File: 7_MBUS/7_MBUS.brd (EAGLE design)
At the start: 67.4 x 44.8 mm, 23 parts, among them T1 BCP51-16, T2 BC847, T3 BC847, X1 AKL18X-02W, X12 ALLSERIALD

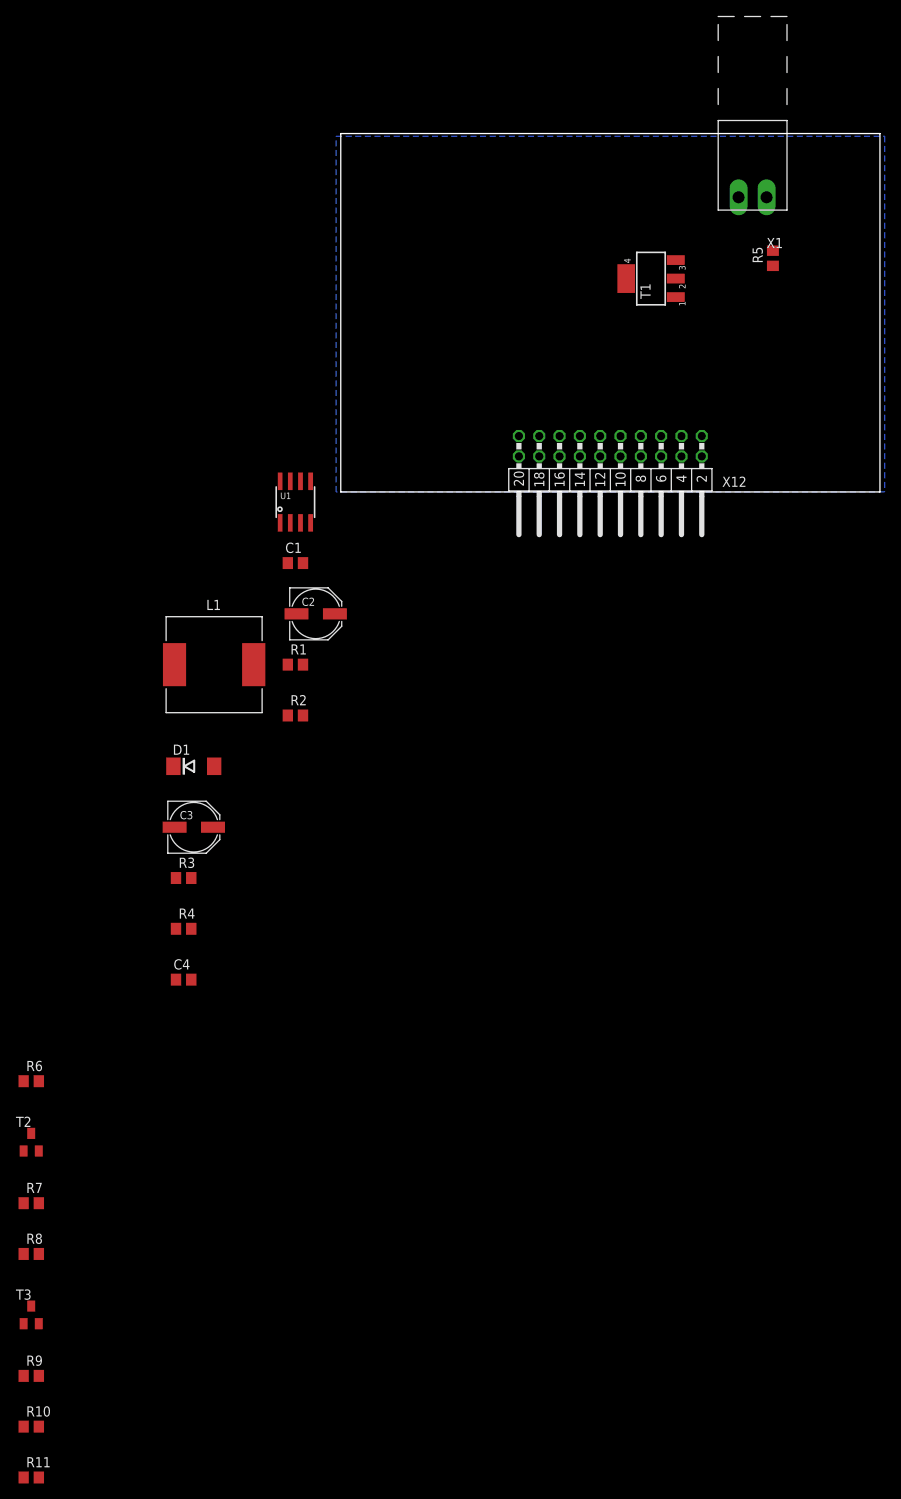
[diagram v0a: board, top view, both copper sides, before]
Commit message: change diodes
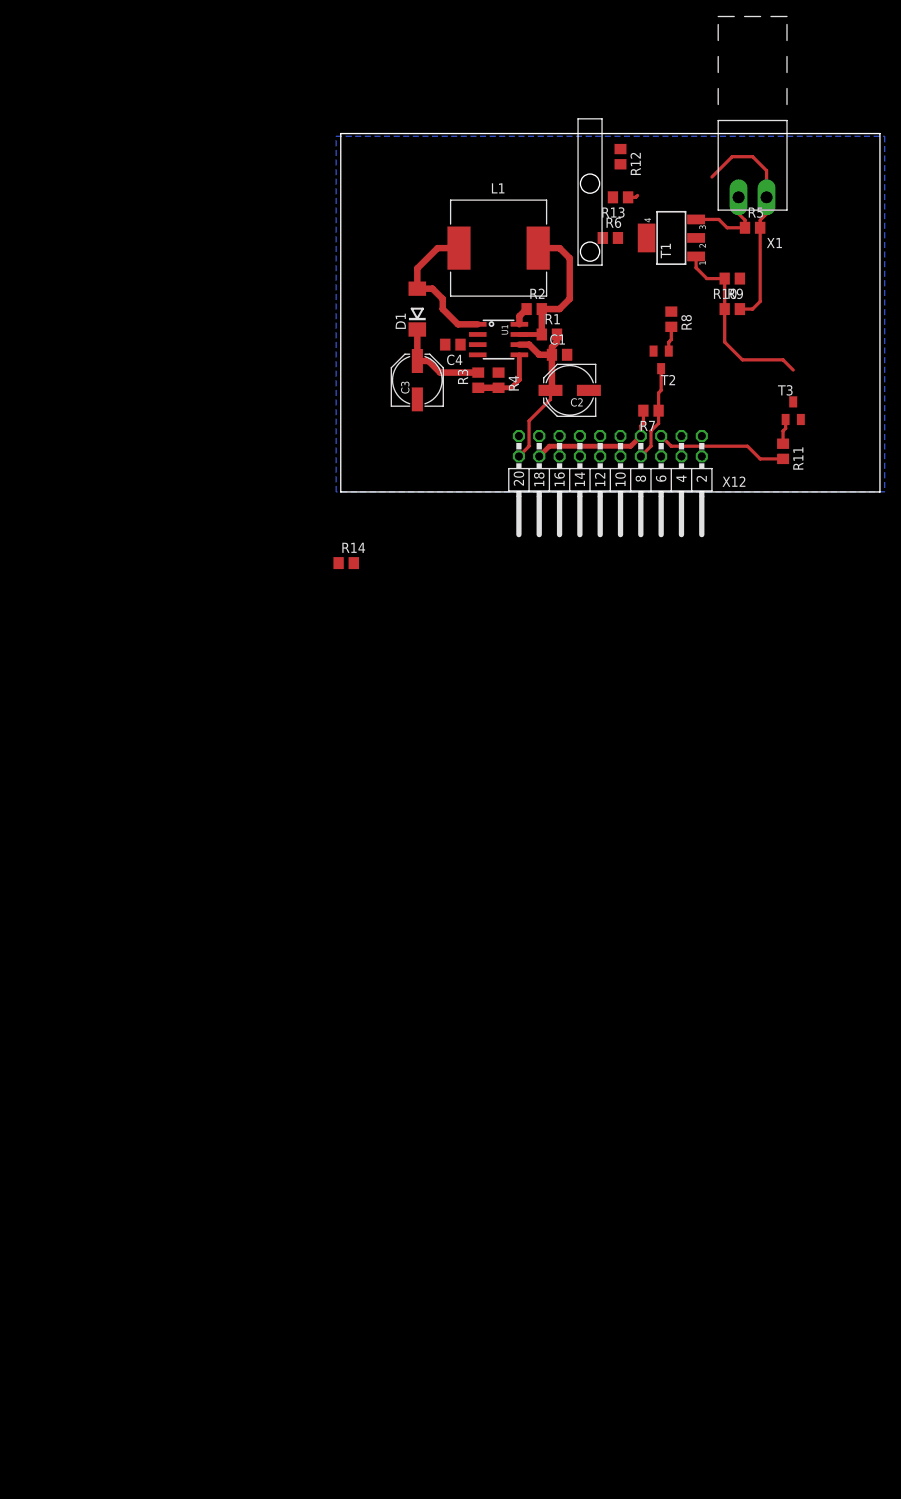
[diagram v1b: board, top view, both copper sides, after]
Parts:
- added R12: 39k, rcl:R0805
- added R13: 22, rcl:R0805
- added R14: 2k2, rcl:R0805
- added U$1: (no value), Mentor:1271.1000
- moved R10 168.1 mm to (15.2, 26.7), turned to 180 degrees
- moved R9 159.6 mm to (15.2, 22.9)
- moved R11 159.0 mm to (21.6, 5.08), turned to 270 degrees
- moved T3 147.8 mm to (22.9, 10.2)
- moved R8 141.6 mm to (7.62, 21.6), turned to 270 degrees
- moved R6 127.9 mm to (0.00, 31.8)
- moved R7 125.8 mm to (5.08, 10.2), turned to 180 degrees
- moved T2 125.6 mm to (6.35, 16.5), turned to 180 degrees
- moved C4 86.2 mm to (-19.7, 18.4), turned to 180 degrees
- moved R4 79.1 mm to (-14.0, 14.0), turned to 270 degrees
- moved R3 72.3 mm to (-16.5, 14.0), turned to 90 degrees
- moved D1 63.6 mm to (-24.1, 22.9), turned to 90 degrees
- moved L1 63.1 mm to (-14.0, 30.5)
- moved C3 62.5 mm to (-24.1, 14.0), turned to 90 degrees
- moved R2 58.9 mm to (-9.53, 22.9)
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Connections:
- new net N$100: R5.2, R9.2, X1.P$1
- new net N$11: R13.1
- new net N$14: R14.2, T3.3
- net 36V: now also R13.2; no longer R5.2, R9.2, X1.P$1
- net GND: now also R12.1; no longer R6.1
- net N$12: now also R14.1; no longer T3.3
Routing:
- net N$100: track 0.00 -> 28.2 mm
- net N$12: track 0.00 -> 23.5 mm
- net +12V: track 0.00 -> 21.8 mm
- net N$2: track 0.00 -> 19.5 mm
- net N$1: track 0.00 -> 18.9 mm
- net +5V: track 0.00 -> 17.1 mm
- net N$8: track 0.00 -> 16.4 mm
- net 36V: track 0.00 -> 12.2 mm
- net N$9: track 0.00 -> 12.0 mm
- net N$7: track 0.00 -> 10.7 mm
- net N$6: track 0.00 -> 8.67 mm
- net N$10: track 0.00 -> 3.16 mm
- net N$13: track 0.00 -> 3.16 mm
- net N$3: track 0.00 -> 2.28 mm
- net N$11: track 0.00 -> 1.28 mm
